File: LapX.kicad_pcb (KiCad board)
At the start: 2 copper layers, 89 x 63 mm, 83 parts, among them J1 Conn_01x12, J2 Conn_02x01, J3 USB_C_Receptacle_PowerOnly_6P, J4 Micro_SD_Card_Det2, Q1 BSS138, Q2 BSS138, Q3 BSS138, Q4 BSS138, U1 TCMT4100, U2 TCMT4100

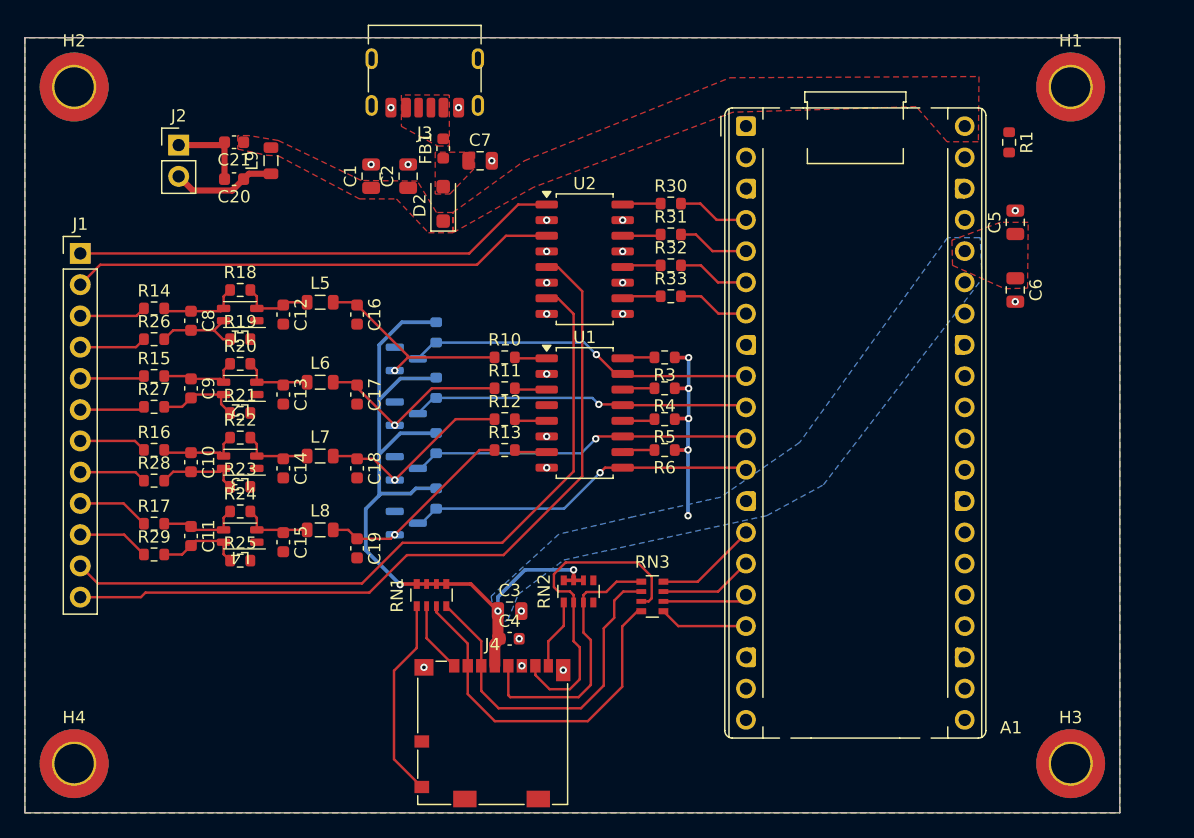
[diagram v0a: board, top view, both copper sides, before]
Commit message: Ärbet
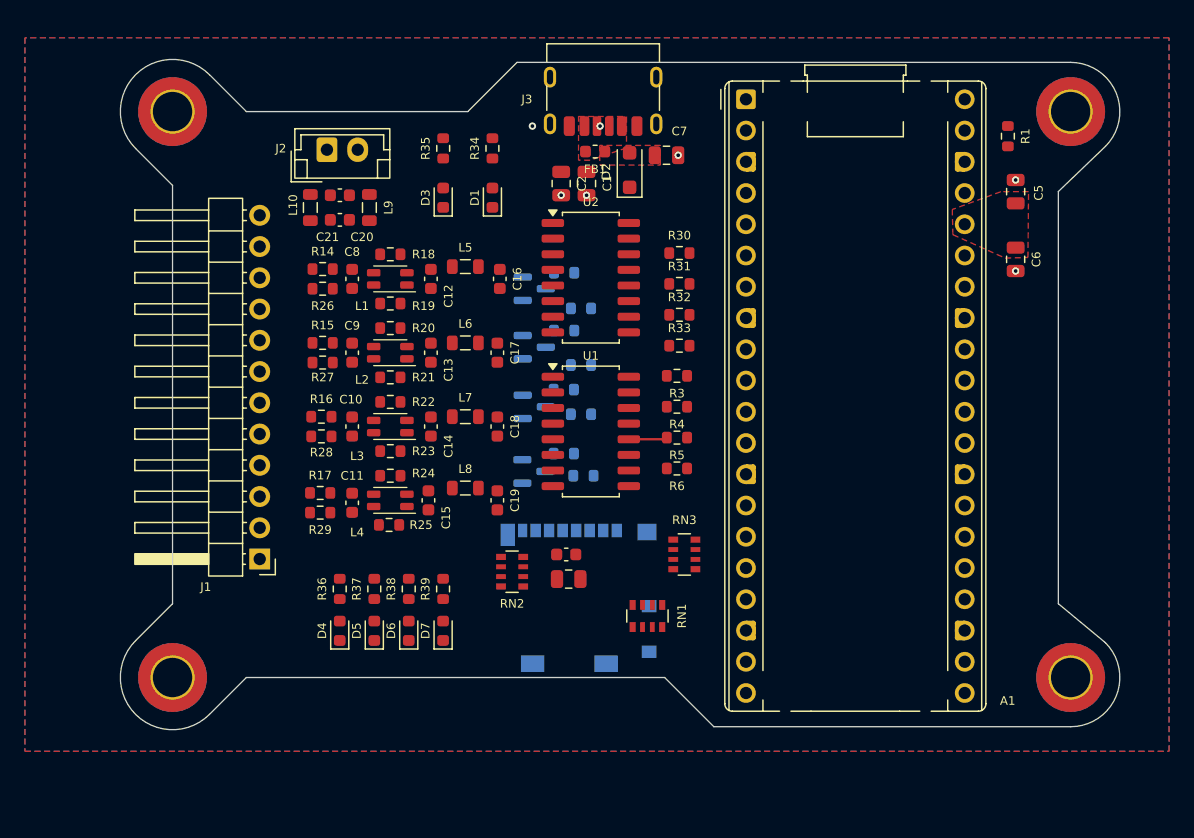
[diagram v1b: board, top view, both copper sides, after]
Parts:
- added D1: LED, LED_SMD:LED_0603_1608Metric, F.Cu at (153.0, 65.0)
- added D3: LED, LED_SMD:LED_0603_1608Metric, F.Cu at (149.0, 65.0)
- added D4: LED, LED_SMD:LED_0603_1608Metric, F.Cu at (140.6, 100.2)
- added D5: LED, LED_SMD:LED_0603_1608Metric, F.Cu at (143.4, 100.2)
- added D6: LED, LED_SMD:LED_0603_1608Metric, F.Cu at (146.2, 100.2)
- added D7: LED, LED_SMD:LED_0603_1608Metric, F.Cu at (149.0, 100.2)
- added L10: 1u, Inductor_SMD:L_0805_2012Metric, F.Cu at (138.2, 65.8)
- added R34: 120, Resistor_SMD:R_0603_1608Metric, F.Cu at (153.0, 61.0)
- added R35: 330, Resistor_SMD:R_0603_1608Metric, F.Cu at (149.0, 61.0)
- added R36: 120, Resistor_SMD:R_0603_1608Metric, F.Cu at (140.6, 96.8)
- added R37: 120, Resistor_SMD:R_0603_1608Metric, F.Cu at (143.4, 96.8)
- added R38: 120, Resistor_SMD:R_0603_1608Metric, F.Cu at (146.2, 96.8)
- added R39: 120, Resistor_SMD:R_0603_1608Metric, F.Cu at (149.0, 96.8)
- J1: footprint Connector_PinHeader_2.54mm:PinHeader_1x12_P2.54mm_Vertical -> Connector_PinHeader_2.54mm:PinHeader_1x12_P2.54mm_Horizontal
- J2: footprint Connector_PinHeader_2.54mm:PinHeader_1x02_P2.54mm_Vertical -> Connector_JST:JST_EH_B2B-EH-A_1x02_P2.50mm_Vertical
- J4, R10, R11, R12, R13: moved to B.Cu
- moved J1 28.8 mm to (134.1, 94.4), turned to 180 degrees
- moved RN1 17.6 mm to (165.6, 99.0), turned to -90 degrees
- moved C1 17.5 mm to (160.7, 63.9), turned to -90 degrees
- moved D2 15.4 mm to (164.2, 62.8)
- moved C7 15.2 mm to (167.2, 61.5)
- moved J3 14.6 mm to (162.0, 56.0)
- moved R26 14.3 mm to (139.2, 72.4)
- moved R27 14.2 mm to (139.2, 78.4)
- moved R14 14.1 mm to (139.2, 70.8)
- moved R28 14.1 mm to (139.1, 84.4)
- moved R15 14.0 mm to (139.2, 76.8)
- moved R29 13.9 mm to (139.0, 90.6)
- moved R16 13.9 mm to (139.1, 82.8)
- moved R17 13.7 mm to (139.0, 89.0)
- moved C8 13.5 mm to (141.6, 71.6)
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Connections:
- net /INPUT_OPTO/CHANNEL_1_PICO renamed /CHANNEL_1_PICO
- net /INPUT_OPTO/CHANNEL_2_PICO renamed /CHANNEL_2_PICO
- net /INPUT_OPTO/CHANNEL_3_PICO renamed /CHANNEL_3_PICO
- net /INPUT_OPTO/CHANNEL_4_PICO renamed /CHANNEL_4_PICO
- A1 pad 25: unconnected-(A1-GPIO19-Pad25) -> /DEBUG_LED1
- A1 pad 26: unconnected-(A1-GPIO20-Pad26) -> /DEBUG_LED2
- A1 pad 27: unconnected-(A1-GPIO21-Pad27) -> /DEBUG_LED3
- A1 pad 29: unconnected-(A1-GPIO22-Pad29) -> /DEBUG_LED4
- C21 pad 2: /VSS_OUT -> GND
- J1 pad 1: /RELAIS_1 -> /RELAIS_3
- J1 pad 10: /INPUT_FILTER/CH4_INPUT_N -> /INPUT_FILTER/CH1_INPUT_P
- J1 pad 11: /RELAIS_4 -> /RELAIS_2
- J1 pad 12: /RELAIS_3 -> /RELAIS_1
- J1 pad 2: /RELAIS_2 -> /RELAIS_4
- J1 pad 3: /INPUT_FILTER/CH1_INPUT_P -> /INPUT_FILTER/CH4_INPUT_N
- J1 pad 4: /INPUT_FILTER/CH1_INPUT_N -> /INPUT_FILTER/CH4_INPUT_P
- J1 pad 5: /INPUT_FILTER/CH2_INPUT_P -> /INPUT_FILTER/CH3_INPUT_N
- J1 pad 6: /INPUT_FILTER/CH2_INPUT_N -> /INPUT_FILTER/CH3_INPUT_P
- J1 pad 7: /INPUT_FILTER/CH3_INPUT_P -> /INPUT_FILTER/CH2_INPUT_N
- J1 pad 8: /INPUT_FILTER/CH3_INPUT_N -> /INPUT_FILTER/CH2_INPUT_P
- J1 pad 9: /INPUT_FILTER/CH4_INPUT_P -> /INPUT_FILTER/CH1_INPUT_N
- RN1 pad 1: /NU_DET1 -> /MOSI
- RN1 pad 2: /NU_DAT2 -> /~{CS}
- RN1 pad 3: /~{CS} -> /NU_DAT2
- RN1 pad 4: /MOSI -> /NU_DET1
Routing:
- net +3.3V: track 83.7 -> 0.00 mm, vias 8 -> 0
- net /RELAIS_3: track 63.6 -> 0.00 mm
- net /RELAIS_4: track 60.0 -> 0.00 mm
- net /RELAIS_2: track 39.6 -> 0.00 mm
- net /RELAIS_1: track 39.6 -> 0.00 mm
- net /~{CS}: track 29.8 -> 0.00 mm
- net /MOSI: track 29.1 -> 0.00 mm
- net /CHANNEL_4_PICO: track 28.6 -> 0.00 mm, vias 1 -> 0
- net /CHANNEL_1_PICO: track 28.4 -> 0.00 mm, vias 1 -> 0
- net /CHANNEL_3_PICO: track 27.8 -> 0.00 mm, vias 1 -> 0
- net /CHANNEL_2_PICO: track 27.5 -> 0.00 mm, vias 1 -> 0
- net /MISO: track 26.7 -> 0.00 mm
- net /CLK: track 22.3 -> 0.00 mm
- net /INPUT_FILTER/CH_1_FILT_OUT: track 16.6 -> 0.00 mm, vias 1 -> 0
- net /NU_DET1: track 16.4 -> 0.00 mm
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- removed copper zone on B.Cu, net +3.3V
- removed copper zone on F.Cu, net VBUS
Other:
- board size 89 x 63 mm -> 81.2 x 54.5 mm
